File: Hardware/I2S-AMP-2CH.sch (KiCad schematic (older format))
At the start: 19 parts, among them U6 TAS5760MDCAR

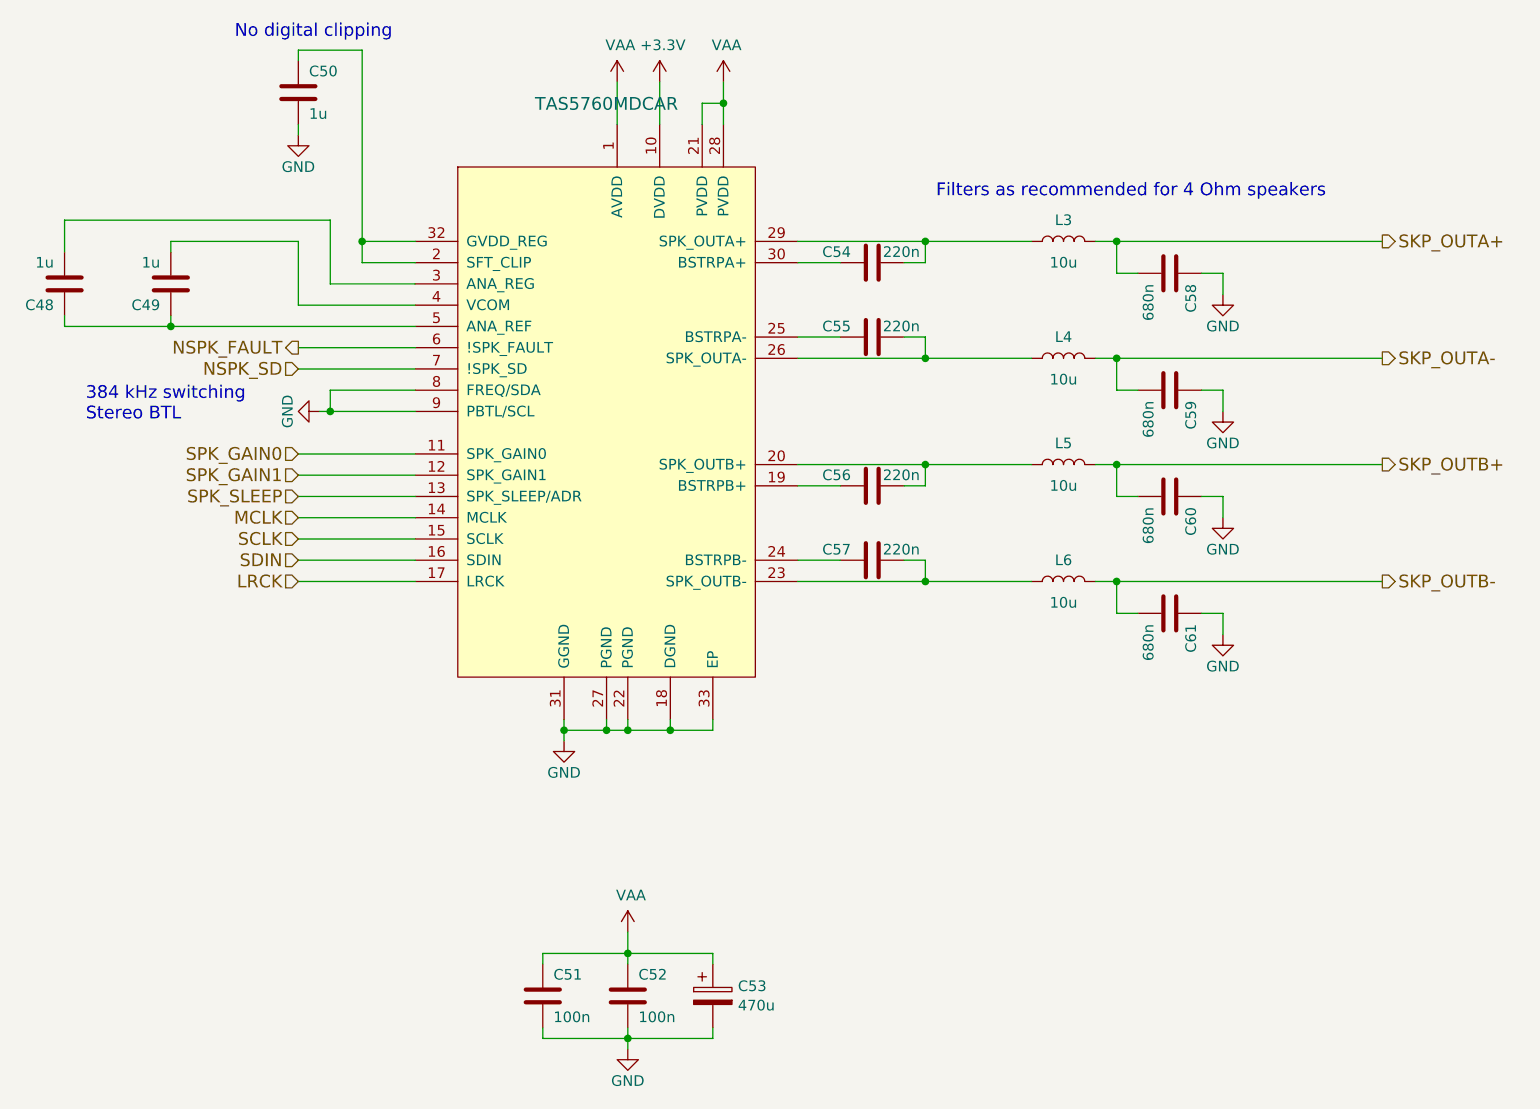
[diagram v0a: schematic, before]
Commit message: hardware bugfixes
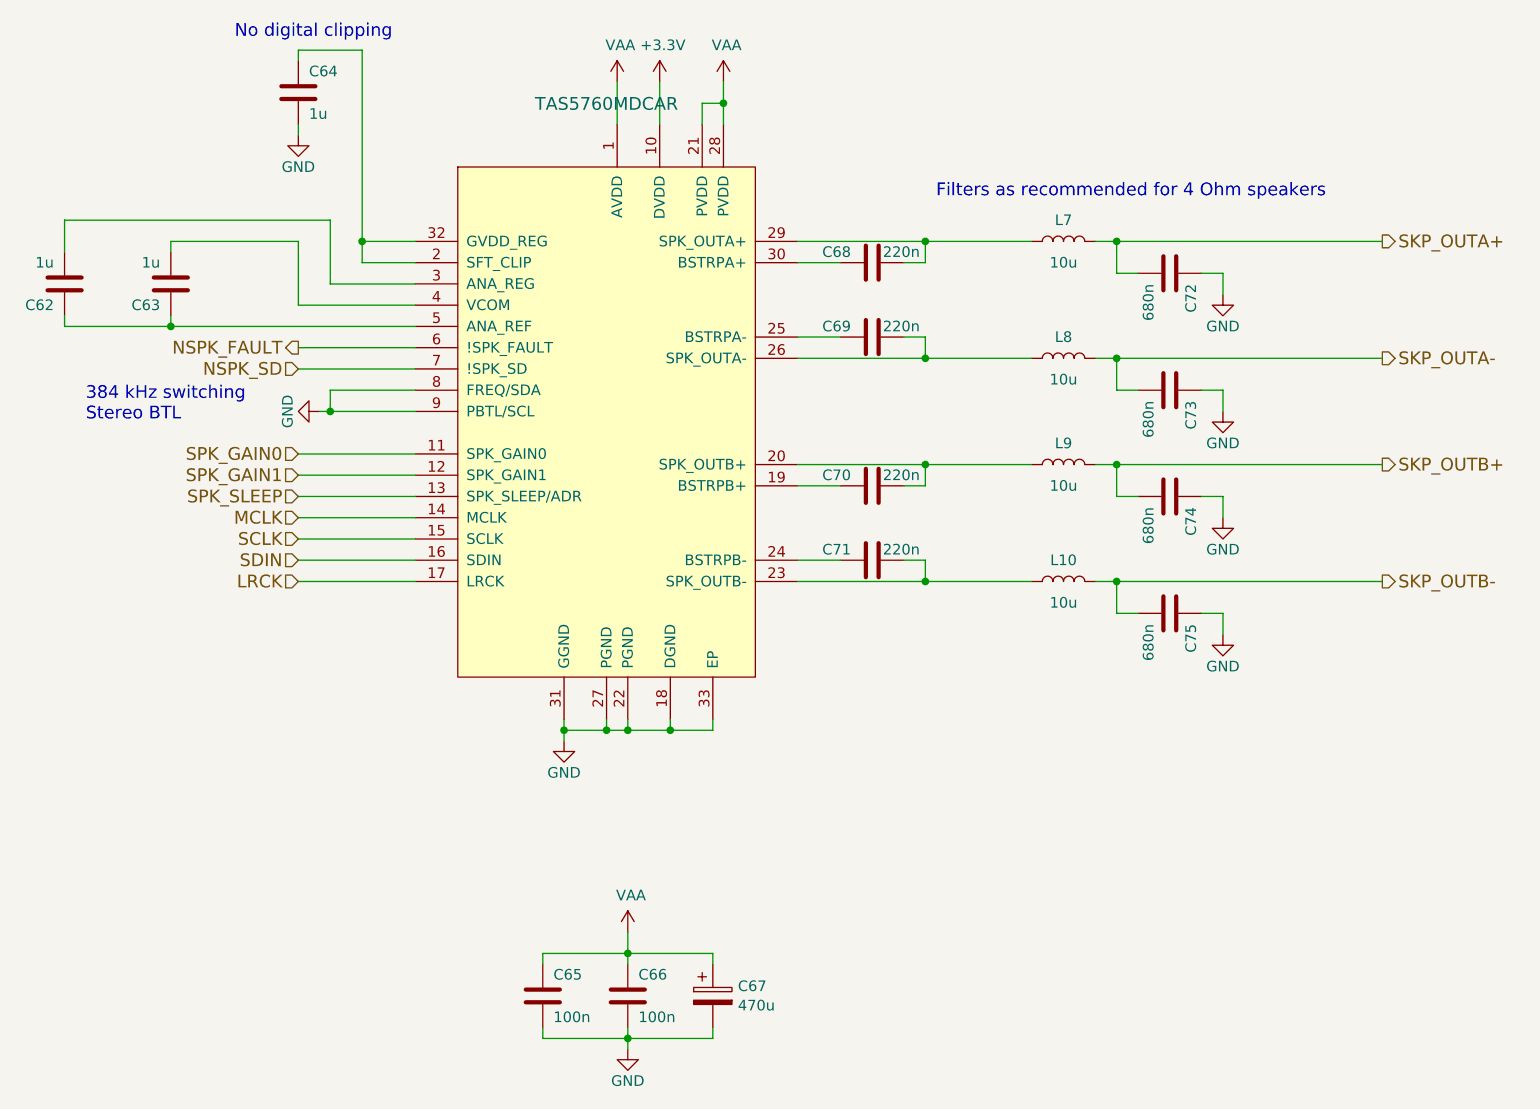
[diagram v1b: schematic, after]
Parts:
- C58, C59, C60, C61: footprint Capacitor_SMD:C_0603_1608Metric_Pad1.08x0.95mm_HandSolder -> Capacitor_SMD:C_0805_2012Metric_Pad1.18x1.45mm_HandSolder
- renumbered U6 to U7

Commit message: various bugfixes
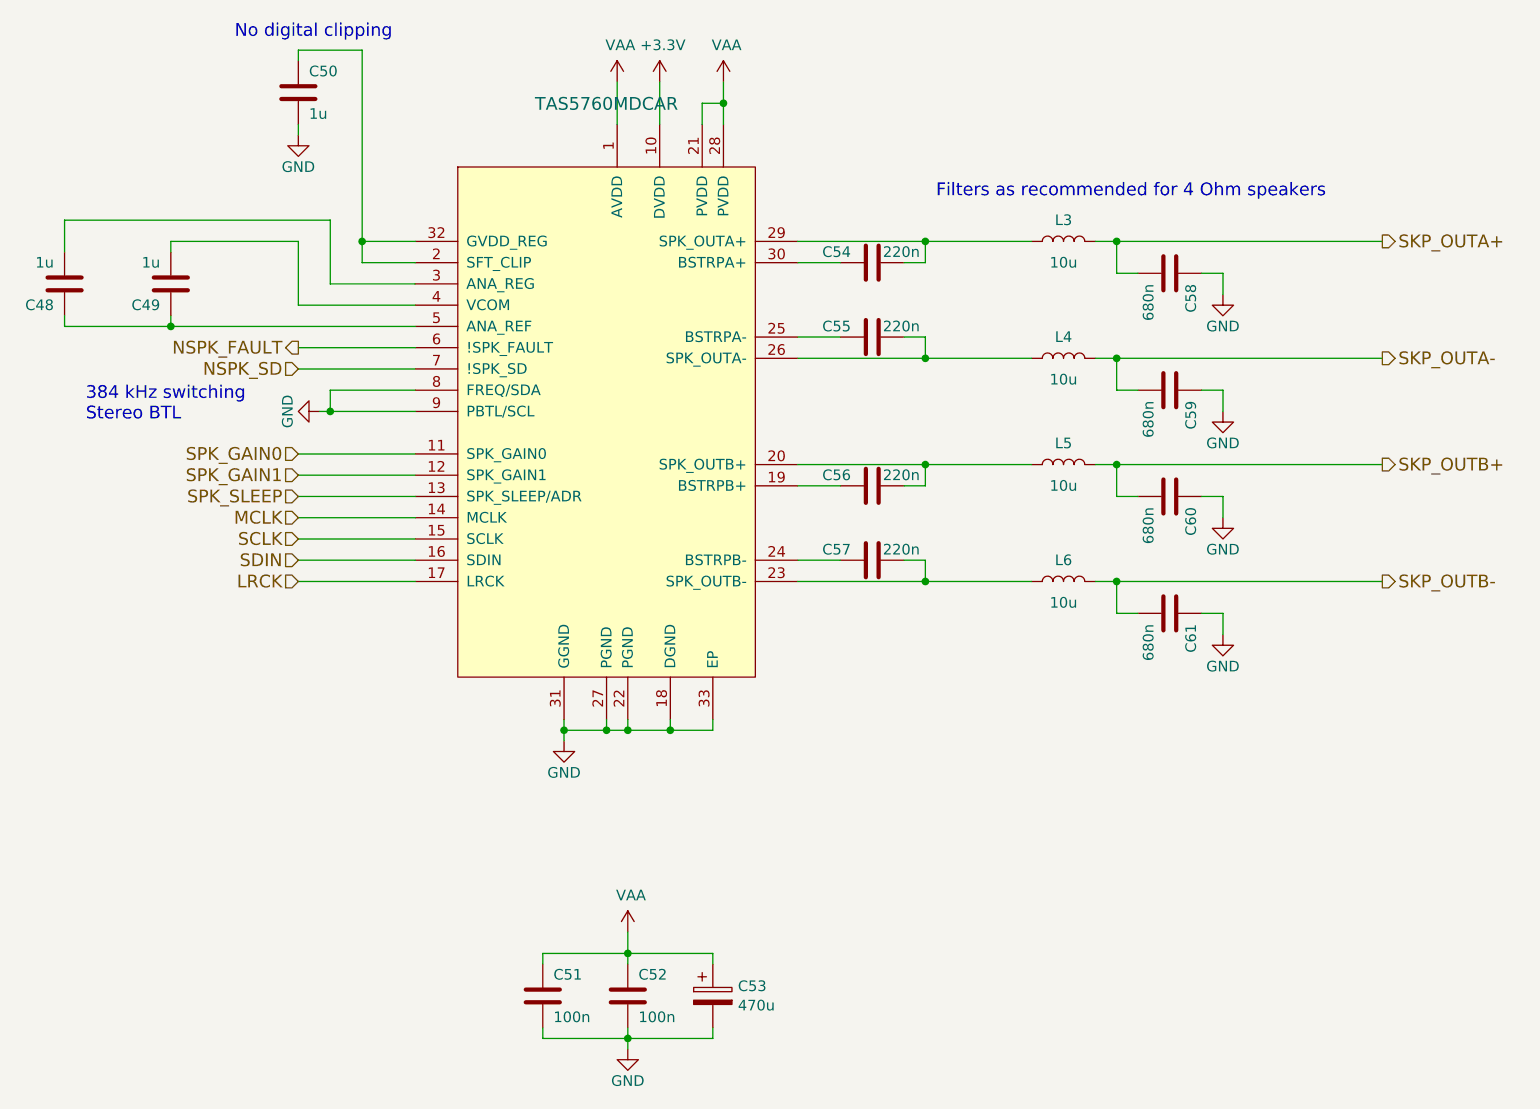
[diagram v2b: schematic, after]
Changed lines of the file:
@@
 $Descr A4 11693 8268
 encoding utf-8
-Sheet 5 8
+Sheet 4 8
 Title "AMP"
 Date "2021-03-30"
@@
 AR Path="/5AF9FF80/574C11BE" Ref="C50"  Part="1"
 AR Path="/608A6138/574C11BE" Ref="C64"  Part="1"
-F 0 "C64" H 3000 1750 50  0000 L CNN
+F 0 "C50" H 3000 1750 50  0000 L CNN
 F 1 "1u" H 3000 1550 50  0000 L CNN
 F 2 "Capacitor_SMD:C_0805_2012Metric_Pad1.18x1.45mm_HandSolder" V 2650 1790 50  0001 C CNN
@@
 AR Path="/5AF9FF80/5B067CFE" Ref="C49"  Part="1"
 AR Path="/608A6138/5B067CFE" Ref="C63"  Part="1"
-F 0 "C63" H 2400 2650 50  0000 L CNN
+F 0 "C49" H 2400 2650 50  0000 L CNN
 F 1 "1u" H 2400 2450 50  0000 L CNN
 F 2 "Capacitor_SMD:C_0805_2012Metric_Pad1.18x1.45mm_HandSolder" V 2050 2690 50  0001 C CNN
@@
 AR Path="/5AF9FF80/5B067CFF" Ref="C48"  Part="1"
 AR Path="/608A6138/5B067CFF" Ref="C62"  Part="1"
-F 0 "C62" H 1900 2650 50  0000 L CNN
+F 0 "C48" H 1900 2650 50  0000 L CNN
 F 1 "1u" H 1900 2450 50  0000 L CNN
 F 2 "Capacitor_SMD:C_0805_2012Metric_Pad1.18x1.45mm_HandSolder" V 1550 2690 50  0001 C CNN
@@
 AR Path="/5AF9FF80/574C26C6" Ref="C52"  Part="1"
 AR Path="/608A6138/574C26C6" Ref="C66"  Part="1"
-F 0 "C66" H 4550 6000 50  0000 L CNN
+F 0 "C52" H 4550 6000 50  0000 L CNN
 F 1 "100n" H 4550 5800 50  0000 L CNN
 F 2 "Capacitor_SMD:C_0603_1608Metric_Pad1.08x0.95mm_HandSolder" V 4200 6040 50  0001 C CNN
@@
 AR Path="/5AF9FF80/5B067D0D" Ref="C57"  Part="1"
 AR Path="/608A6138/5B067D0D" Ref="C71"  Part="1"
-F 0 "C71" V 5700 3950 50  0000 L CNN
+F 0 "C57" V 5700 3950 50  0000 L CNN
 F 1 "220n" V 5700 3800 50  0000 R CNN
 F 2 "Capacitor_SMD:C_0603_1608Metric_Pad1.08x0.95mm_HandSolder" V 5350 3990 50  0001 C CNN
@@
 AR Path="/5AF9FF80/5B067D11" Ref="C55"  Part="1"
 AR Path="/608A6138/5B067D11" Ref="C69"  Part="1"
-F 0 "C69" V 5700 2900 50  0000 L CNN
+F 0 "C55" V 5700 2900 50  0000 L CNN
 F 1 "220n" V 5700 2750 50  0000 R CNN
 F 2 "Capacitor_SMD:C_0603_1608Metric_Pad1.08x0.95mm_HandSolder" V 5350 2940 50  0001 C CNN
@@
 AR Path="/5AF9FF80/5B067D13" Ref="C54"  Part="1"
 AR Path="/608A6138/5B067D13" Ref="C68"  Part="1"
-F 0 "C68" V 5700 2550 50  0000 L CNN
+F 0 "C54" V 5700 2550 50  0000 L CNN
 F 1 "220n" V 5700 2400 50  0000 R CNN
 F 2 "Capacitor_SMD:C_0603_1608Metric_Pad1.08x0.95mm_HandSolder" V 5350 2590 50  0001 C CNN
@@
 AR Path="/5AF9FF80/6097B2F1" Ref="C53"  Part="1"
 AR Path="/608A6138/6097B2F1" Ref="C67"  Part="1"
-F 0 "C67" H 5018 5946 50  0000 L CNN
+F 0 "C53" H 5018 5946 50  0000 L CNN
 F 1 "470u" H 5018 5855 50  0000 L CNN
 F 2 "Capacitor_THT:CP_Radial_D16.0mm_P7.50mm" H 4938 5750 50  0001 C CNN
@@
 AR Path="/5AF9FF80/60988667" Ref="C51"  Part="1"
 AR Path="/608A6138/60988667" Ref="C65"  Part="1"
-F 0 "C65" H 4150 6000 50  0000 L CNN
+F 0 "C51" H 4150 6000 50  0000 L CNN
 F 1 "100n" H 4150 5800 50  0000 L CNN
 F 2 "Capacitor_SMD:C_0603_1608Metric_Pad1.08x0.95mm_HandSolder" V 3800 6040 50  0001 C CNN
@@
 AR Path="/5AF9FF80/5B067D14" Ref="L3"  Part="1"
 AR Path="/608A6138/5B067D14" Ref="L7"  Part="1"
-F 0 "L7" V 6650 2350 50  0000 C CNN
+F 0 "L3" V 6650 2350 50  0000 C CNN
 F 1 "10u" V 6450 2350 50  0000 C CNN
 F 2 "Inductor_SMD:L_Abracon_ASPI-0630LR" H 6550 2350 50  0001 C CNN
@@
 AR Path="/5AF9FF80/60D816DE" Ref="L4"  Part="1"
 AR Path="/608A6138/60D816DE" Ref="L8"  Part="1"
-F 0 "L8" V 6650 2900 50  0000 C CNN
+F 0 "L4" V 6650 2900 50  0000 C CNN
 F 1 "10u" V 6450 2900 50  0000 C CNN
 F 2 "Inductor_SMD:L_Abracon_ASPI-0630LR" H 6550 2900 50  0001 C CNN
@@
 AR Path="/5AF9FF80/60D87D8D" Ref="L5"  Part="1"
 AR Path="/608A6138/60D87D8D" Ref="L9"  Part="1"
-F 0 "L9" V 6650 3400 50  0000 C CNN
+F 0 "L5" V 6650 3400 50  0000 C CNN
 F 1 "10u" V 6450 3400 50  0000 C CNN
 F 2 "Inductor_SMD:L_Abracon_ASPI-0630LR" H 6550 3400 50  0001 C CNN
@@
 AR Path="/5AF9FF80/60D87DA0" Ref="L6"  Part="1"
 AR Path="/608A6138/60D87DA0" Ref="L10"  Part="1"
-F 0 "L10" V 6650 3950 50  0000 C CNN
+F 0 "L6" V 6650 3950 50  0000 C CNN
 F 1 "10u" V 6450 3950 50  0000 C CNN
 F 2 "Inductor_SMD:L_Abracon_ASPI-0630LR" H 6550 3950 50  0001 C CNN
@@
 AR Path="/5AF9FF80/5B067D19" Ref="C58"  Part="1"
 AR Path="/608A6138/5B067D19" Ref="C72"  Part="1"
-F 0 "C72" H 7100 2600 50  0000 L CNN
+F 0 "C58" H 7100 2600 50  0000 L CNN
 F 1 "680n" H 7100 2400 50  0000 L CNN
 F 2 "Capacitor_SMD:C_0805_2012Metric_Pad1.18x1.45mm_HandSolder" V 6750 2640 50  0001 C CNN
@@
 AR Path="/5AF9FF80/60D9BA43" Ref="C59"  Part="1"
 AR Path="/608A6138/60D9BA43" Ref="C73"  Part="1"
-F 0 "C73" H 7100 3150 50  0000 L CNN
+F 0 "C59" H 7100 3150 50  0000 L CNN
 F 1 "680n" H 7100 2950 50  0000 L CNN
 F 2 "Capacitor_SMD:C_0805_2012Metric_Pad1.18x1.45mm_HandSolder" V 6750 3190 50  0001 C CNN
@@
 AR Path="/5AF9FF80/60D9DAD3" Ref="C60"  Part="1"
 AR Path="/608A6138/60D9DAD3" Ref="C74"  Part="1"
-F 0 "C74" H 7100 3650 50  0000 L CNN
+F 0 "C60" H 7100 3650 50  0000 L CNN
 F 1 "680n" H 7100 3450 50  0000 L CNN
 F 2 "Capacitor_SMD:C_0805_2012Metric_Pad1.18x1.45mm_HandSolder" V 6750 3690 50  0001 C CNN
@@
 AR Path="/5AF9FF80/60D9FB44" Ref="C61"  Part="1"
 AR Path="/608A6138/60D9FB44" Ref="C75"  Part="1"
-F 0 "C75" H 7100 4200 50  0000 L CNN
+F 0 "C61" H 7100 4200 50  0000 L CNN
 F 1 "680n" H 7100 4000 50  0000 L CNN
 F 2 "Capacitor_SMD:C_0805_2012Metric_Pad1.18x1.45mm_HandSolder" V 6750 4240 50  0001 C CNN
@@
 AR Path="/5AF9FF80/60C136E8" Ref="C56"  Part="1"
 AR Path="/608A6138/60C136E8" Ref="C70"  Part="1"
-F 0 "C70" V 5700 3600 50  0000 L CNN
+F 0 "C56" V 5700 3600 50  0000 L CNN
 F 1 "220n" V 5700 3450 50  0000 R CNN
 F 2 "Capacitor_SMD:C_0603_1608Metric_Pad1.08x0.95mm_HandSolder" V 5350 3640 50  0001 C CNN
@@
 AR Path="/5AF9FF80/608A7BF7" Ref="U7"  Part="1"
 AR Path="/608A6138/608A7BF7" Ref="U8"  Part="1"
-F 0 "U8" H 4400 5150 60  0001 C TNN
+F 0 "U7" H 4400 5150 60  0001 C TNN
 F 1 "TAS5760MDCAR" H 4400 4697 60  0000 C CNN
 F 2 "Package_SO:HTSSOP-32-1EP_6.1x11mm_P0.65mm_EP5.2x11mm_Mask4.11x4.36mm_ThermalVias" H 4300 3100 60  0001 C CNN
